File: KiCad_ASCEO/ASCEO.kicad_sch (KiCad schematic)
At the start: 25 parts, among them J1 USB_OTG, J2 JST-XH 6-Pin (To Motor + Enco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, J3 JST-XH 5-Pin (To Raspberry Pi), J4 Barrel_Jack, J5 Screw_Terminal, SW1 RESET1, SW2 BOOT1, U1 ESP32-S3-WROOM-1-N4, U2 LDI1117-3.3H

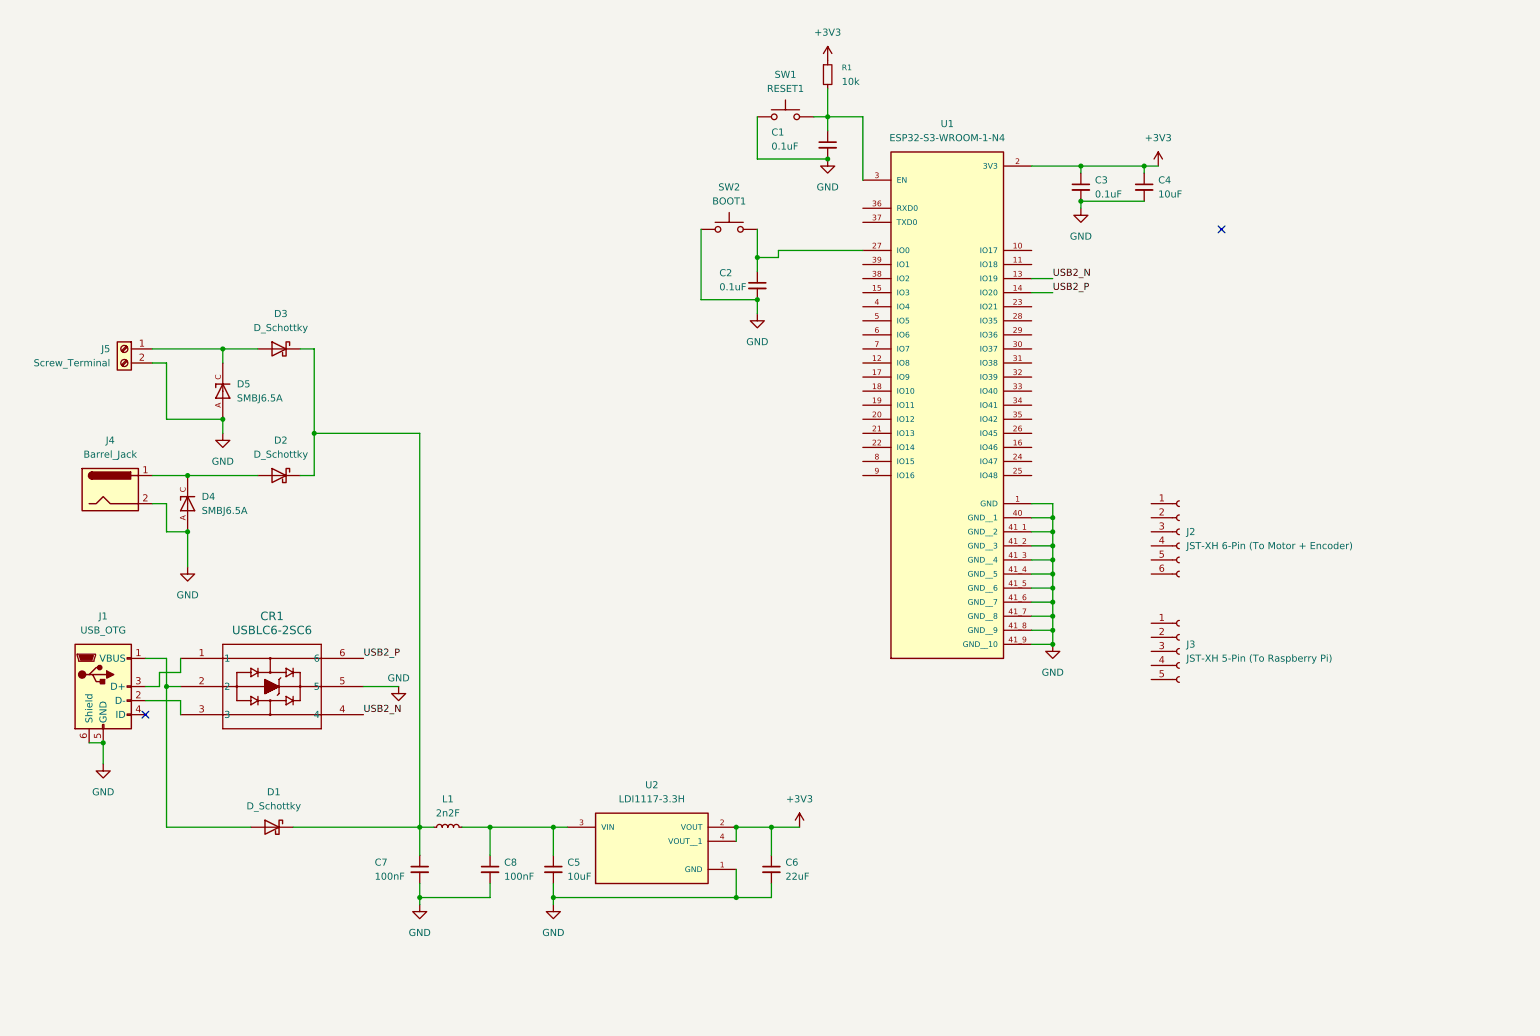
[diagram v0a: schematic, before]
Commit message: First Draft Schematic
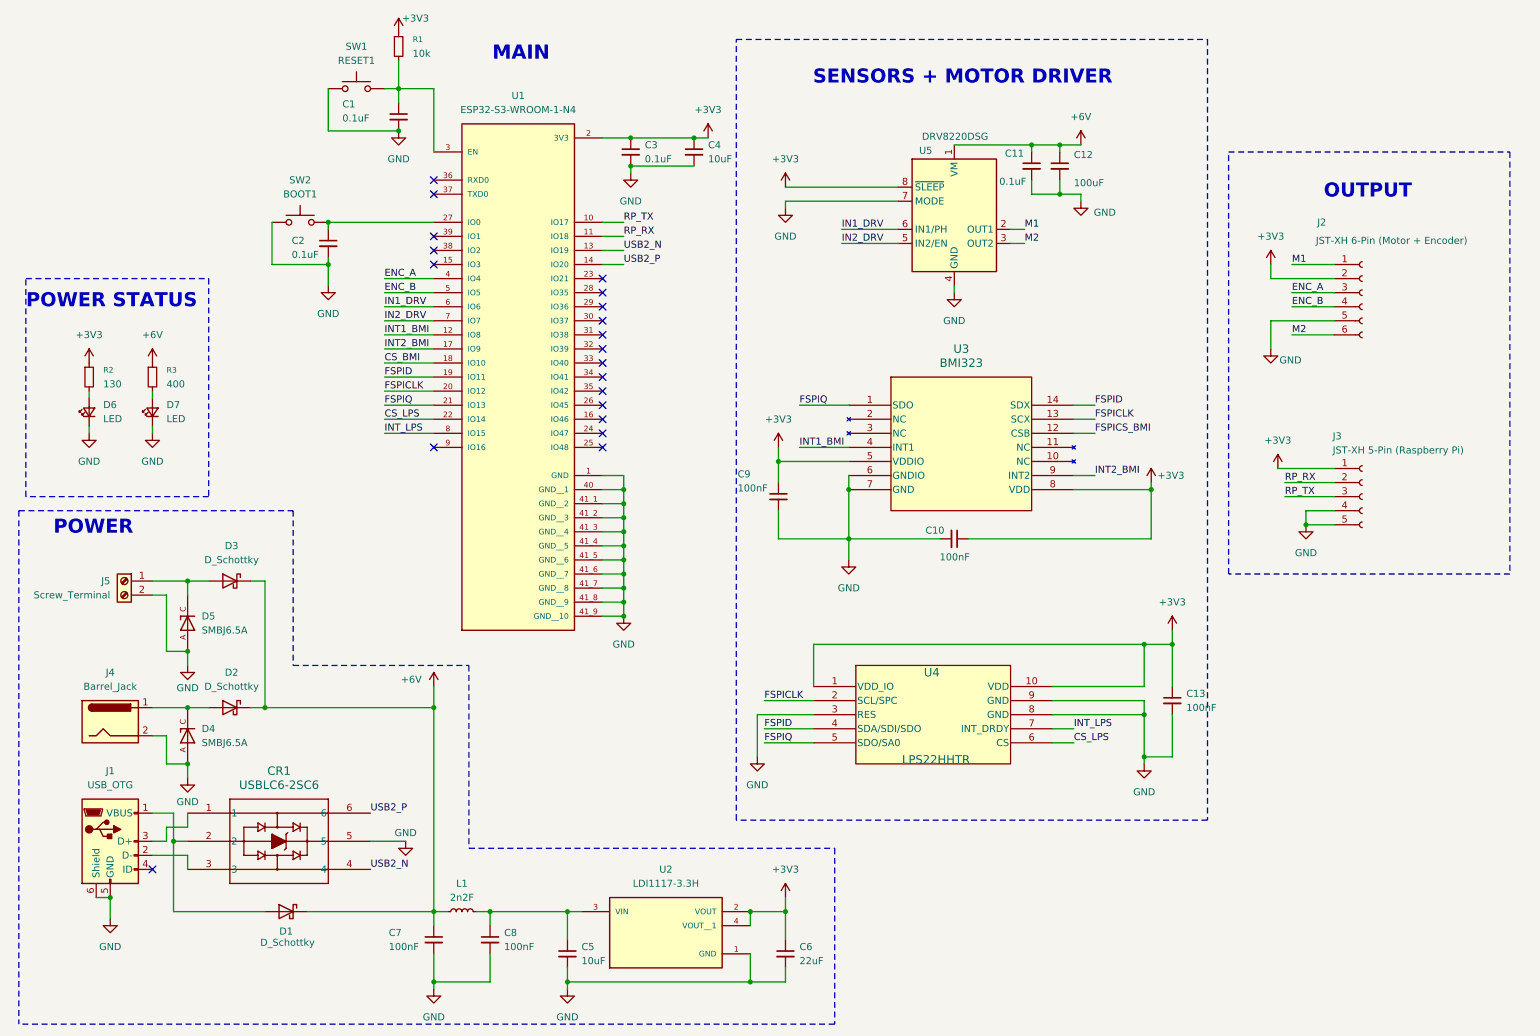
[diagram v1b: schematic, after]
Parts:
- added C10, C13, C9: 100nF, symbol Device:C_Small
- added C11: 0.1uF, symbol Device:C_Small
- added C12: 100uF, symbol Device:C_Small
- added D6, D7: LED, symbol Device:LED_Small
- added R2: 130, symbol Device:R_Small
- added R3: 400, symbol Device:R_Small
- added U3: BMI323, BMI323_BOS, symbol BMI323:BMI323
- added U4: LPS22HHTR, HLGA-10L_2X2X0P73_STM, symbol LPS22HHTR:LPS22HHTR
- added U5: DRV8220DSG, Package_SON:WSON-8-1EP_2x2mm_P0.5mm_EP0.9x1.6mm, symbol Driver_Motor:DRV8220DSG
- J2: value JST-XH 6-Pin (To Motor + Encoder) -> JST-XH 6-Pin (Motor + Encoder)
- J3: value JST-XH 5-Pin (To Raspberry Pi) -> JST-XH 5-Pin (Raspberry Pi)
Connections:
- net +3V3: now also J2.2 (Pin_2), J3.1 (Pin_1), C10.1, C13.1, C9.1, R2.1, U3.5 (VDDIO), U3.8 (VDD), U4.1 (VDD_IO), U4.10 (VDD), U5.8 (~{SLEEP})
- net GND: now also J2.5 (Pin_5), J3.4 (Pin_4), J3.5 (Pin_5), C10.2, C11.2, C12.2, C13.2, C9.2, D6.1 (K), D7.1 (K), U3.6 (GNDIO), U3.7 (GND), U4.3 (RES), U4.8 (GND), U4.9 (GND), U5.4 (GND), U5.7 (MODE), U5.9 (GND)
- net +6V: now reaches C7.1, D1.1 (K), D2.1 (K), D3.1 (K), L1.1
- net +6V: now also C11.1, C12.1, R3.1, U5.1 (VM)
- net RP_RX: now reaches J3.2 (Pin_2)
- net RP_RX: now also U1.11 (IO18)
- net RP_TX: now reaches J3.3 (Pin_3)
- net RP_TX: now also U1.10 (IO17)
- net INT1_BMI: now reaches U1.12 (IO8)
- net INT1_BMI: now also U3.4 (INT1)
- net INT2_BMI: now reaches U1.17 (IO9)
- net INT2_BMI: now also U3.9 (INT2)
- net CS_BMI: now reaches U1.18 (IO10)
- net FSPID: now reaches U1.19 (IO11)
- net FSPID: now also U3.14 (SDX), U4.4 (SDA/SDI/SDO)
- net FSPICLK: now reaches U1.20 (IO12)
- net FSPICLK: now also U3.13 (SCX), U4.2 (SCL/SPC)
- net FSPIQ: now reaches U1.21 (IO13)
- net FSPIQ: now also U3.1 (SDO), U4.5 (SDO/SA0)
- net CS_LPS: now reaches U1.22 (IO14)
- net CS_LPS: now also U4.6 (CS)
- net ENC_A: now reaches U1.4 (IO4)
- net ENC_A: now also J2.3 (Pin_3)
- net ENC_B: now reaches U1.5 (IO5)
- net ENC_B: now also J2.4 (Pin_4)
- net IN1_DRV: now reaches U1.6 (IO6)
- net IN1_DRV: now also U5.6 (IN1/PH)
- net IN2_DRV: now reaches U1.7 (IO7)
- net IN2_DRV: now also U5.5 (IN2/EN)
- net INT_LPS: now reaches U1.8 (IO15)
- net INT_LPS: now also U4.7 (INT_DRDY)
- net M1: now reaches J2.1 (Pin_1)
- net M1: now also U5.2 (OUT1)
- net M2: now reaches J2.6 (Pin_6)
- net M2: now also U5.3 (OUT2)
- new net: D6.2 (A), R2.2
- new net: D7.2 (A), R3.2
- new net FSPICS_BMI: U3.12 (CSB)
- no-connect marks 2 -> 20
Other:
- note added: "MAIN"
- note added: "OUTPUT"
- note added: "POWER"
- note added: "POWER STATUS"
- note added: "SENSORS + MOTOR DRIVER"
- moved on the sheet: C1, C2, C3, C4, C5, C6, C7, C8, CR1, D1, D2, D3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

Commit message: Footprint Refresh
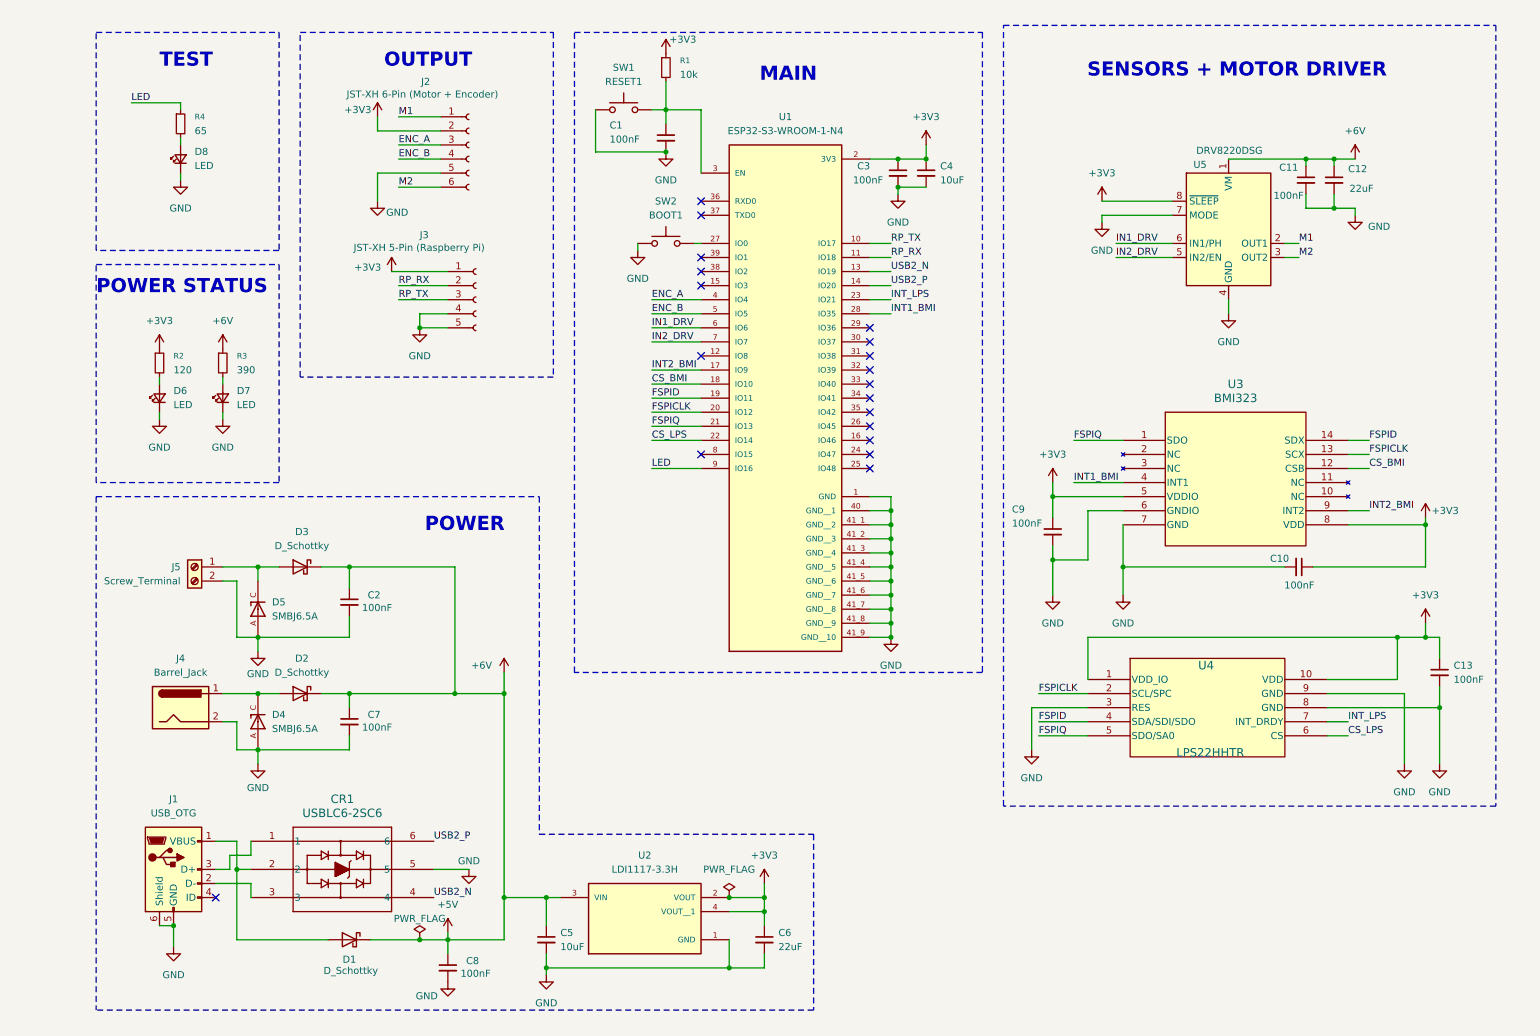
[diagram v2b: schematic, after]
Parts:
- removed L1: 2n2F, symbol Device:L_Small
- added D8: LED, LED_SMD:LED_0805_2012Metric_Pad1.15x1.40mm_HandSolder, symbol Device:LED_Small
- added R4: 65, Resistor_SMD:R_0603_1608Metric_Pad0.98x0.95mm_HandSolder, symbol Device:R_Small
- C1, C11, C2, C3: value 0.1uF -> 100nF; footprint (none) -> Capacitor_SMD:C_0805_2012Metric_Pad1.18x1.45mm_HandSolder
- C10, C13, C4, C5, C7, C8, C9: footprint (none) -> Capacitor_SMD:C_0805_2012Metric_Pad1.18x1.45mm_HandSolder
- C12: value 100uF -> 22uF; footprint (none) -> Capacitor_THT:CP_Radial_D12.5mm_P5.00mm
- C6: footprint (none) -> Capacitor_THT:CP_Radial_D12.5mm_P5.00mm
- CR1: footprint SOT23-6L_STM -> USBLC6:SOT23-6L_STM
- D1, D2, D3: footprint (none) -> Diode_SMD:D_SMA_Handsoldering
- D6, D7: footprint (none) -> LED_SMD:LED_0805_2012Metric_Pad1.15x1.40mm_HandSolder
- J1: footprint (none) -> USB-miniB675031020:CON00317_5_MOL
- J4: footprint (none) -> PJ-073:SAMESKY_PJ-073
- J5: footprint (none) -> CUI_TB002:CUI_TB002-500-02BE
- R1: footprint (none) -> Resistor_SMD:R_0805_2012Metric_Pad1.20x1.40mm_HandSolder
- R2: value 130 -> 120; footprint (none) -> Resistor_SMD:R_0603_1608Metric_Pad0.98x0.95mm_HandSolder
- R3: value 400 -> 390; footprint (none) -> Resistor_SMD:R_0603_1608Metric_Pad0.98x0.95mm_HandSolder
- SW1, SW2: footprint (none) -> SWT0210:SW_SWT0210-045026GSA_REVA
- U3: footprint BMI323_BOS -> BMI323:BMI323_BOS
- U4: footprint HLGA-10L_2X2X0P73_STM -> LPS22HHTR:HLGA-10L_2X2X0P73_STM
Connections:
- net +6V is gone; now on net +5V: C11.1, C12.1, C7.1, D1.1 (K), D2.1 (K), D3.1 (K), R3.1, U5.1 (VM)
- net FSPICS_BMI is gone; now on net CS_BMI: U3.12 (CSB)
- net GND: now also D8.1 (K)
- net INT1_BMI: now also U1.28 (IO35); no longer U1.12 (IO8)
- net INT_LPS: now also U1.23 (IO21); no longer U1.8 (IO15)
- net +5V: now reaches C5.1, C8.1, U2.3 (VIN)
- net +5V: now also C2.1
- net at SW2.2, U1.27 (IO0): no longer C2.1
- net LED: now reaches U1.9 (IO16)
- net LED: now also R4.1
- new net: D8.2 (A), R4.2
- no-connect marks 20 -> 19
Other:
- note added: "TEST"
- moved on the sheet: C1, C10, C11, C12, C13, C3, C4, C5, C6, C9, CR1, D1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
